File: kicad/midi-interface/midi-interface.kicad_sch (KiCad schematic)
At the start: 3 parts, among them J1 Conn_01x05_Pin, U1 ATmega328P-P, Y1 Crystal

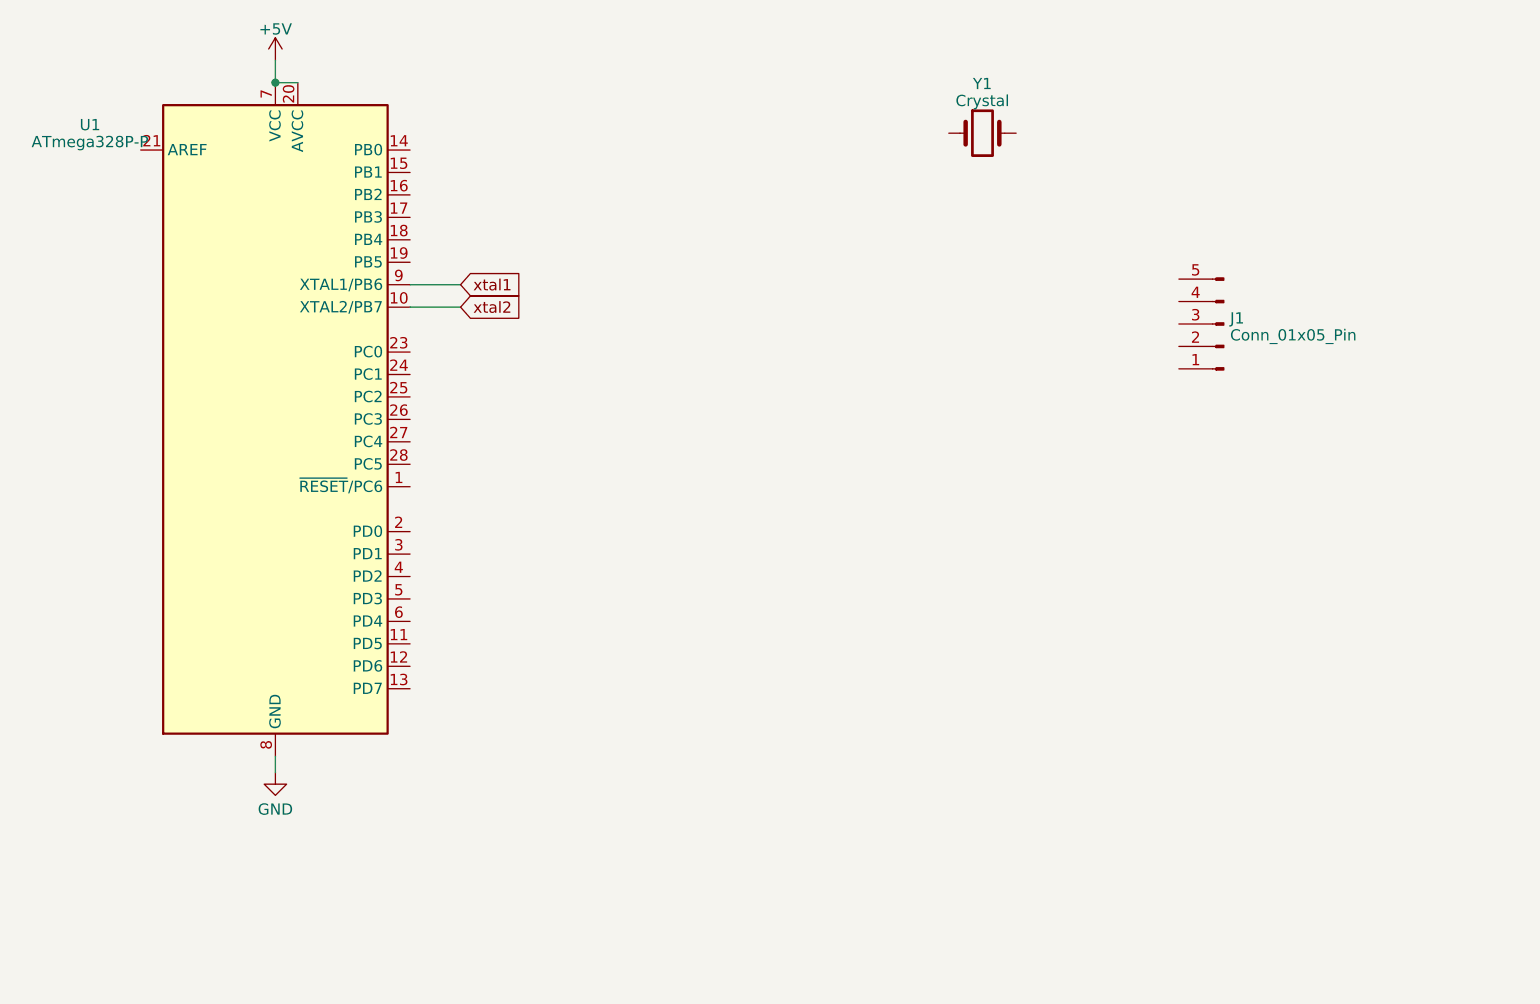
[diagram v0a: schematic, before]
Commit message: midi interface kicad update
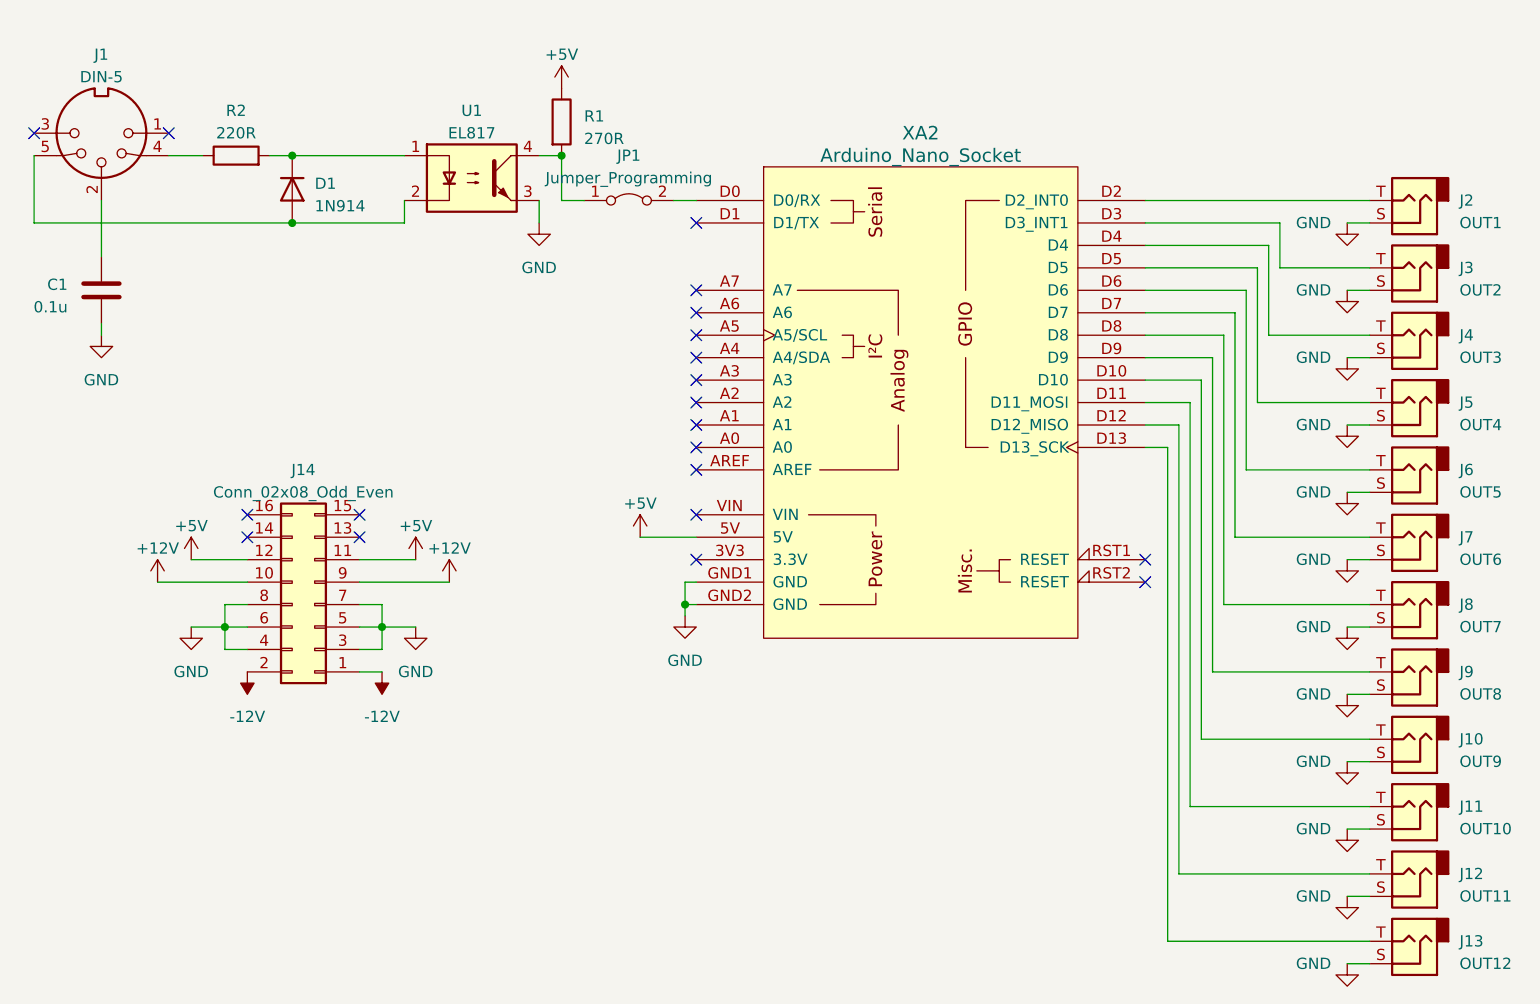
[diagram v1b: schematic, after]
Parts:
- removed J1: Conn_01x05_Pin, symbol Connector:Conn_01x05_Pin
- removed U1: ATmega328P-P, Package_DIP:DIP-28_W7.62mm, symbol MCU_Microchip_ATmega:ATmega328P-P
- removed Y1: Crystal, symbol Device:Crystal
- added C1: 0.1u, Capacitor_SMD:C_1206_3216Metric_Pad1.33x1.80mm_HandSolder, symbol Device:C
- added D1: 1N914, Diode_SMD:D_1206_3216Metric_Pad1.42x1.75mm_HandSolder, symbol Diode:1N914
- added J1: DIN-5, Connector_PinHeader_2.54mm:PinHeader_1x05_P2.54mm_Vertical, symbol Connector:DIN-5_180degree
- added J10: OUT9, Connector_Audio:Jack_3.5mm_QingPu_WQP-PJ398SM_Vertical_CircularHoles, symbol Connector_Audio:AudioJack2
- added J11: OUT10, Connector_Audio:Jack_3.5mm_QingPu_WQP-PJ398SM_Vertical_CircularHoles, symbol Connector_Audio:AudioJack2
- added J12: OUT11, Connector_Audio:Jack_3.5mm_QingPu_WQP-PJ398SM_Vertical_CircularHoles, symbol Connector_Audio:AudioJack2
- added J13: OUT12, Connector_Audio:Jack_3.5mm_QingPu_WQP-PJ398SM_Vertical_CircularHoles, symbol Connector_Audio:AudioJack2
- added J14: Conn_02x08_Odd_Even, Connector_IDC:IDC-Header_2x08_P2.54mm_Vertical, symbol Connector_Generic:Conn_02x08_Odd_Even
- added J2: OUT1, Connector_Audio:Jack_3.5mm_QingPu_WQP-PJ398SM_Vertical_CircularHoles, symbol Connector_Audio:AudioJack2
- added J3: OUT2, Connector_Audio:Jack_3.5mm_QingPu_WQP-PJ398SM_Vertical_CircularHoles, symbol Connector_Audio:AudioJack2
- added J4: OUT3, Connector_Audio:Jack_3.5mm_QingPu_WQP-PJ398SM_Vertical_CircularHoles, symbol Connector_Audio:AudioJack2
- added J5: OUT4, Connector_Audio:Jack_3.5mm_QingPu_WQP-PJ398SM_Vertical_CircularHoles, symbol Connector_Audio:AudioJack2
- added J6: OUT5, Connector_Audio:Jack_3.5mm_QingPu_WQP-PJ398SM_Vertical_CircularHoles, symbol Connector_Audio:AudioJack2
- added J7: OUT6, Connector_Audio:Jack_3.5mm_QingPu_WQP-PJ398SM_Vertical_CircularHoles, symbol Connector_Audio:AudioJack2
- added J8: OUT7, Connector_Audio:Jack_3.5mm_QingPu_WQP-PJ398SM_Vertical_CircularHoles, symbol Connector_Audio:AudioJack2
- added J9: OUT8, Connector_Audio:Jack_3.5mm_QingPu_WQP-PJ398SM_Vertical_CircularHoles, symbol Connector_Audio:AudioJack2
- added JP1: Jumper_Programming, Connector_PinHeader_2.54mm:PinHeader_1x02_P2.54mm_Vertical, symbol Jumper:Jumper_2_Bridged
- added R1: 270R, Resistor_SMD:R_1206_3216Metric_Pad1.30x1.75mm_HandSolder, symbol Device:R
- added R2: 220R, Resistor_SMD:R_1206_3216Metric_Pad1.30x1.75mm_HandSolder, symbol Device:R
- added U1: EL817, Package_DIP:DIP-4_W7.62mm, symbol Isolator:EL817
- added XA2: Arduino_Nano_Socket, arduino:Arduino_Nano_Socket, symbol arduino:Arduino_Nano_Socket
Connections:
- net +5V: now also J14.11 (Pin_11), J14.12 (Pin_12), R1.1, XA2.5V
- net GND: now also C1.1, J10.S, J11.S, J12.S, J13.S, J14.3 (Pin_3), J14.4 (Pin_4), J14.5 (Pin_5), J14.6 (Pin_6), J14.7 (Pin_7), J14.8 (Pin_8), J2.S, J3.S, J4.S, J5.S, J6.S, J7.S, J8.S, J9.S, U1.3, XA2.GND1 (GND), XA2.GND2 (GND)
- new net: J11.T, XA2.D11 (D11_MOSI)
- new net: J2.T, XA2.D2 (D2_INT0)
- new net: J10.T, XA2.D10
- new net: JP1.1 (A), R1.2, U1.4
- new net: J13.T, XA2.D13 (D13_SCK)
- new net: JP1.2 (B), XA2.D0 (D0/RX)
- new net: J12.T, XA2.D12 (D12_MISO)
- new net: J3.T, XA2.D3 (D3_INT1)
- new net: J4.T, XA2.D4
- new net: J5.T, XA2.D5
- new net: J6.T, XA2.D6
- new net: J7.T, XA2.D7
- new net: J8.T, XA2.D8
- new net: J9.T, XA2.D9
- new net: C1.2, J1.2
- new net: J1.4, R2.1
- new net: D1.1 (K), R2.2, U1.1
- new net: D1.2 (A), J1.5, U1.2
- new net +12V: J14.10 (Pin_10), J14.9 (Pin_9)
- new net -12V: J14.1 (Pin_1), J14.2 (Pin_2)
- no-connect marks 0 -> 20
